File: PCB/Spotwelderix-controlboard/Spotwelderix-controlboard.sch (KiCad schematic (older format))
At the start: 47 parts, among them J1 LEDs, J2 ChargerPower, J3 ExtPwr_FAn, J4 Testpin, P1 Display, P2 CONN_01X08, Q1 AO3400A, Q2 AO3400A, Q3 AO3400A, U1 NodeMCU32, U2 LM7805M_TO263

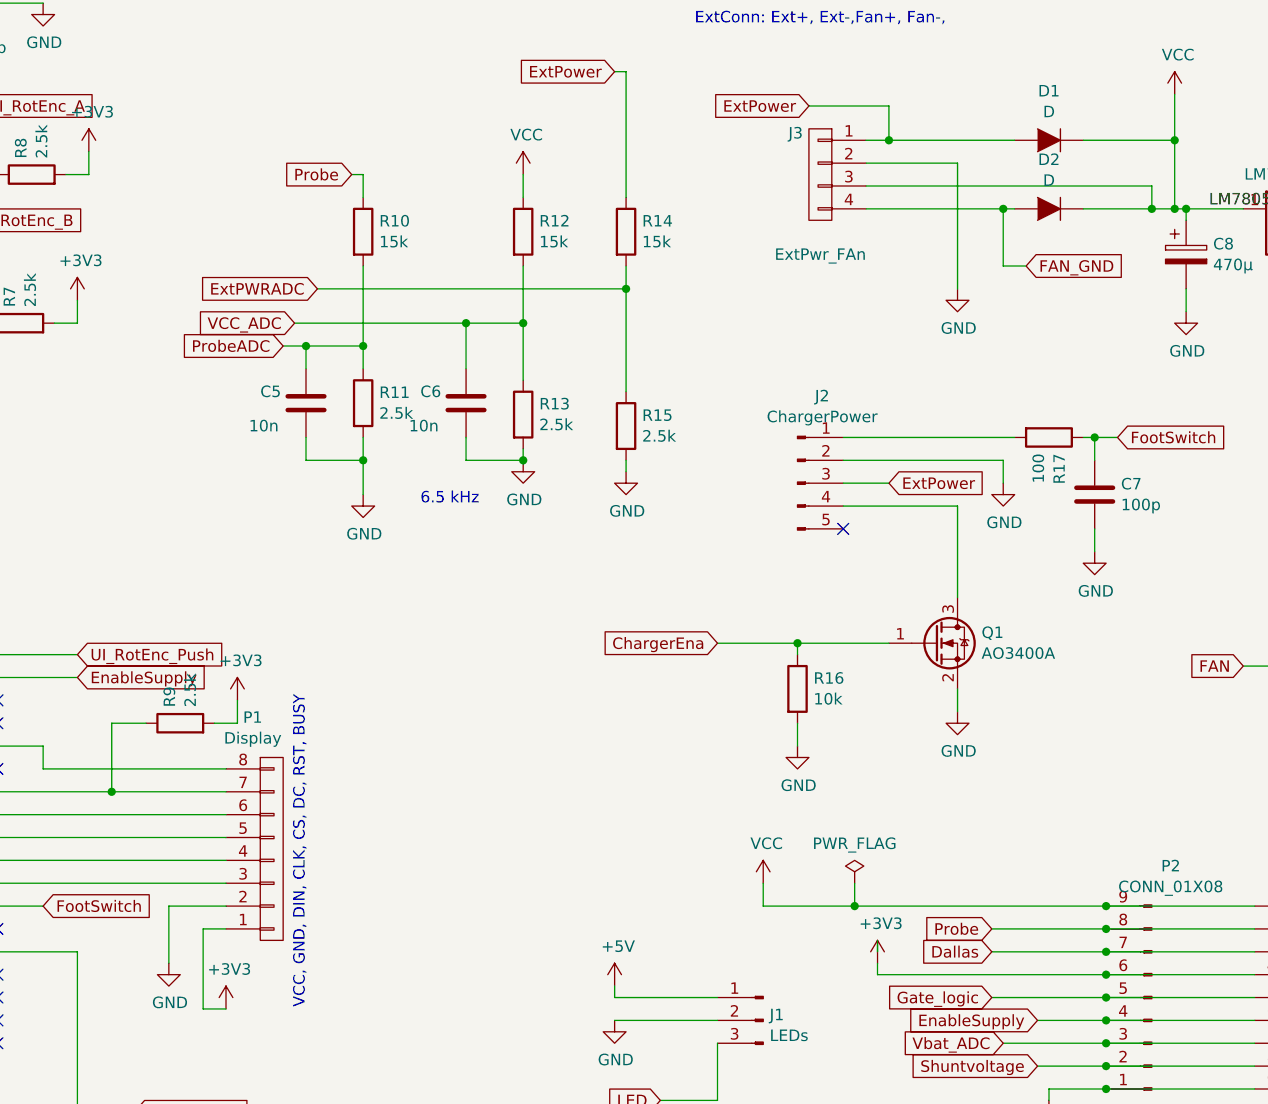
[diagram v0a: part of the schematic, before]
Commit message: clean up
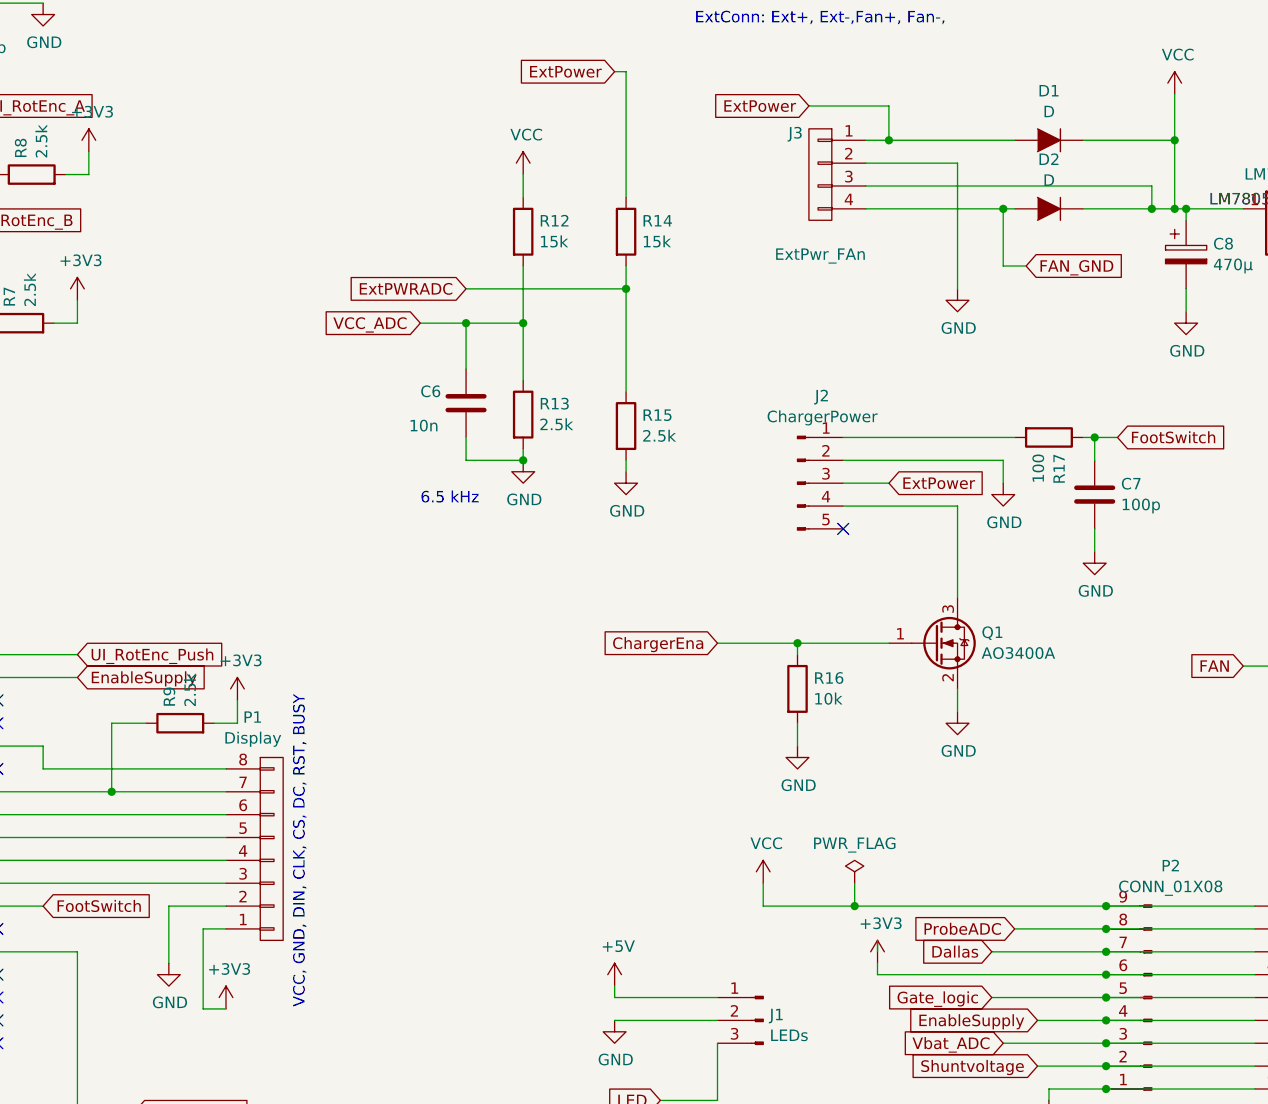
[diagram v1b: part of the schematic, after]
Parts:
- removed C5: 10n, Capacitor_SMD:C_1206_3216Metric_Pad1.33x1.80mm_HandSolder, symbol Spotwelderix-controlboard-rescue:C-Device
- removed R10: 15k, Resistor_SMD:R_0805_2012Metric, symbol Arduino_Spot_Welderparts:R
- removed R11: 2.5k, Resistor_SMD:R_0805_2012Metric, symbol Arduino_Spot_Welderparts:R
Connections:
- net Probe is gone; now on net ProbeADC: J4.2 (Pin_2), P2.8 (Pin_8)
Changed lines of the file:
@@
 	1    0    0    -1
 $EndComp
-Text GLabel 8450 4750 0    50   Input ~ 0
-Probe
-$Comp
-L Arduino_Spot_Welderparts:R R10
-U 1 1 601B227D
-P 5700 1700
-F 0 "R10" H 5770 1746 50  0000 L CNN
-F 1 "15k" H 5770 1655 50  0000 L CNN
-F 2 "Resistor_SMD:R_0805_2012Metric" V 5630 1700 50  0001 C CNN
-F 3 "" H 5700 1700 50  0000 C CNN
-	1    5700 1700
-	1    0    0    -1
-$EndComp
-$Comp
-L Arduino_Spot_Welderparts:R R11
-U 1 1 601B2283
-P 5700 2450
-F 0 "R11" H 5770 2496 50  0000 L CNN
-F 1 "2.5k" H 5770 2405 50  0000 L CNN
-F 2 "Resistor_SMD:R_0805_2012Metric" H 5770 2359 50  0001 L CNN
-F 3 "" H 5700 2450 50  0001 C CNN
-	1    5700 2450
-	1    0    0    -1
-$EndComp
-$Comp
-L Spotwelderix-controlboard-rescue:GND-power #PWR017
-U 1 1 601B2294
-P 5700 2850
-F 0 "#PWR017" H 5700 2600 50  0001 C CNN
-F 1 "GND" H 5705 2677 50  0000 C CNN
-F 2 "" H 5700 2850 50  0001 C CNN
-F 3 "" H 5700 2850 50  0001 C CNN
-	1    5700 2850
-	1    0    0    -1
-$EndComp
-Wire Wire Line
-	5700 2850 5700 2700
-Text GLabel 5650 1450 0    50   Input ~ 0
-Probe
-Wire Wire Line
-	5650 1450 5700 1450
-Wire Wire Line
-	5700 1450 5700 1550
 $Comp
 L Arduino_Spot_Welderparts:CONN_01X04 J3
@@
 Wire Wire Line
 	1450 5450 1450 5550
-Text GLabel 5350 2200 0    50   Input ~ 0
-ProbeADC
-Text GLabel 5400 2100 0    50   Input ~ 0
+Text GLabel 5950 2100 0    50   Input ~ 0
 VCC_ADC
 Connection ~ 6400 2100
-Wire Wire Line
-	5350 2200 5450 2200
-Connection ~ 5700 2200
 Wire Wire Line
 	1750 3600 2150 3600
@@
 Wire Wire Line
 	6400 2100 6400 2350
-Wire Wire Line
-	5700 2200 5700 2300
 $Comp
 L Spotwelderix-controlboard-rescue:NodeMCU32-my_parts U1
@@
 	8650 5150 8950 5150
 Wire Wire Line
-	8450 4750 8950 4750
+	8550 4750 8950 4750
 Wire Wire Line
 	8450 5050 8950 5050
@@
 Text GLabel 8650 5150 0    50   Input ~ 0
 EnableSupply
-Wire Wire Line
-	5700 1850 5700 2200
 Text GLabel 8500 5250 0    50   Input ~ 0
 Vbat_ADC
@@
 Text GLabel 6800 1000 0    50   Input ~ 0
 ExtPower
-Text GLabel 5500 1950 0    50   Input ~ 0
+Text GLabel 6150 1950 0    50   Input ~ 0
 ExtPWRADC
 Wire Wire Line
@@
 Wire Wire Line
 	5000 6850 5150 6850
-$Comp
-L Spotwelderix-controlboard-rescue:C-Device C5
-U 1 1 610D9E59
-P 5450 2450
-F 0 "C5" H 5250 2500 50  0000 L CNN
-F 1 "10n" H 5200 2350 50  0000 L CNN
-F 2 "Capacitor_SMD:C_1206_3216Metric_Pad1.33x1.80mm_HandSolder" H 5488 2300 50  0001 C CNN
-F 3 "https://www.mouser.de/ProductDetail/Samsung-Electro-Mechanics/CL31A106KBHNNNE/?qs=sGAEpiMZZMuMW9TJLBQkXpvci%252BYHLlg21rnqFxf28Ww%3D" H 5450 2450 50  0001 C CNN
-	1    5450 2450
-	1    0    0    -1
-$EndComp
-Wire Wire Line
-	5450 2300 5450 2200
-Connection ~ 5450 2200
-Wire Wire Line
-	5450 2200 5700 2200
-Wire Wire Line
-	5450 2600 5450 2700
-Wire Wire Line
-	5450 2700 5700 2700
-Connection ~ 5700 2700
-Wire Wire Line
-	5700 2700 5700 2600
-Wire Wire Line
-	5500 1950 6850 1950
-Wire Wire Line
-	5400 2100 6150 2100
+Wire Wire Line
+	6150 1950 6850 1950
+Wire Wire Line
+	5950 2100 6150 2100
 $Comp
 L Spotwelderix-controlboard-rescue:C-Device C6
@@
 Wire Wire Line
 	900  4700 1300 4700
+Text GLabel 8550 4750 0    50   Input ~ 0
+ProbeADC
 $EndSCHEMATC
